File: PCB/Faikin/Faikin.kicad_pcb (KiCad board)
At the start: 2 copper layers, 70 x 70 mm, 47 parts, among them J1 1x5, J2 TC2030-USB-NL, J3 Reset, Q1 BSS138PS, U1 TPS562246, U4 ESP32-S3-MINI-1

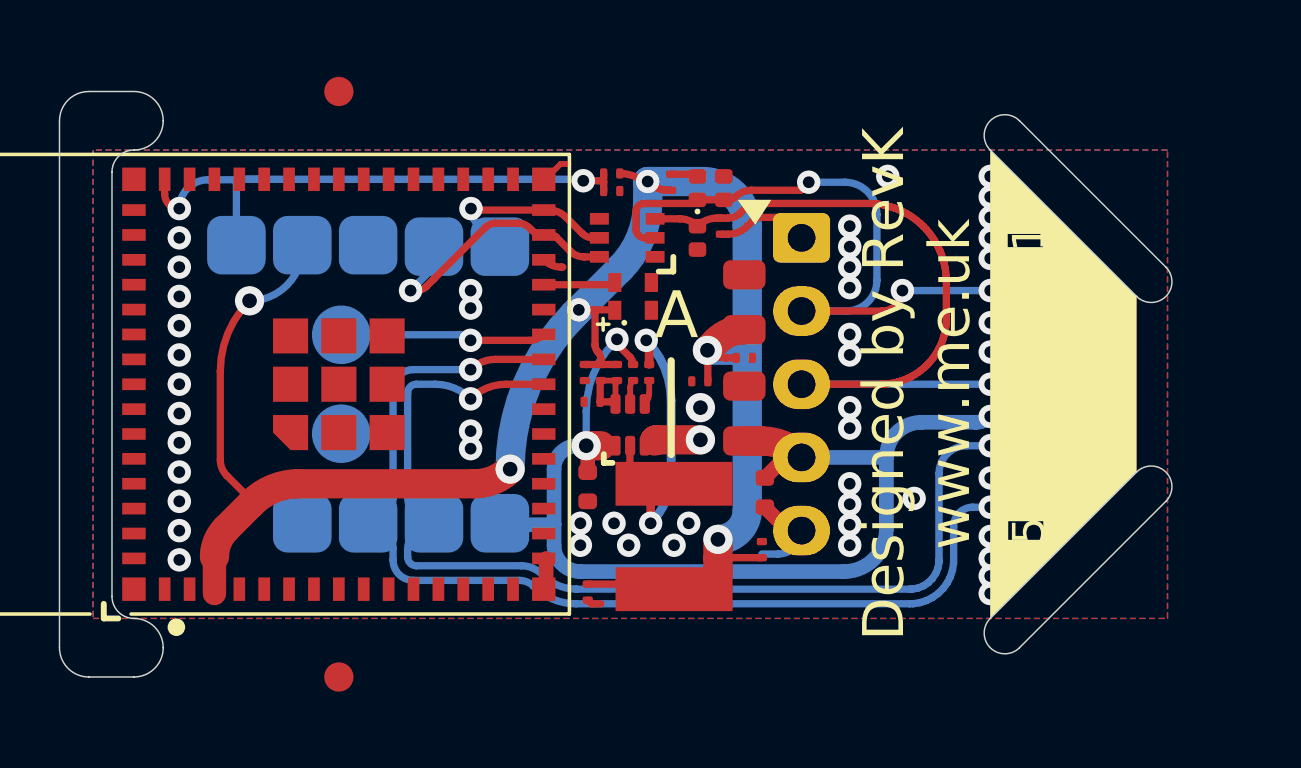
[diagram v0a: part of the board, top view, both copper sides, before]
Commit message: Minor tweaks
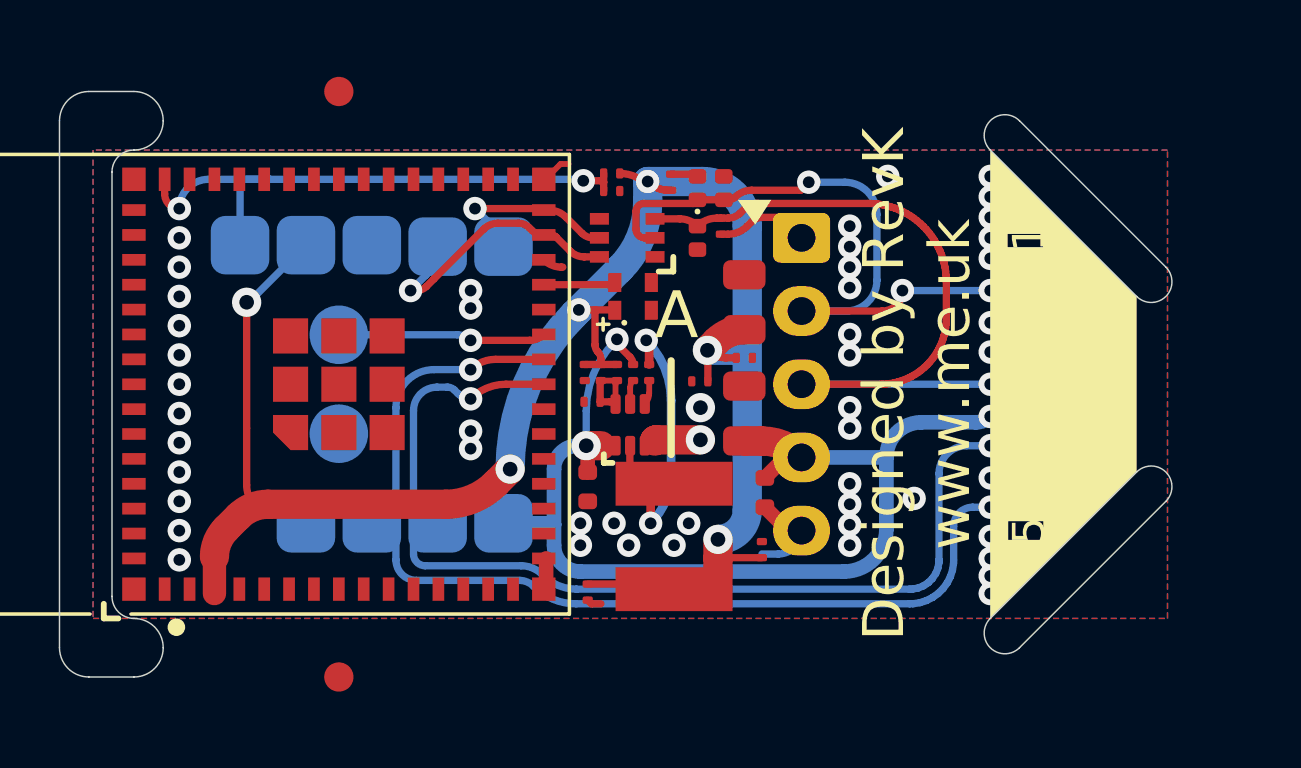
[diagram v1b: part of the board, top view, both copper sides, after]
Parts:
- D1: footprint RevK:SMD1615 -> RevK:SMD1615-Blind
- moved TP10 0.12 mm to (135.4, 60.3)
- moved TP2 0.12 mm to (133.1, 69.8)
- moved TP3 0.12 mm to (130.9, 69.8)
- moved TP4 0.12 mm to (128.6, 69.8)
- moved TP5 0.12 mm to (128.6, 60.2)
- moved TP6 0.12 mm to (126.4, 60.2)
- moved TP7 0.12 mm to (135.4, 69.8)
- moved TP8 0.12 mm to (130.9, 60.2)
- moved TP9 0.12 mm to (133.1, 60.3)
- moved J3 0.08 mm to (129.8, 65.0)
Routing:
- net D-: track 38.9 -> 37.2 mm
- net D+: track 43.7 -> 42.3 mm
- net TX: track 6.23 -> 5.34 mm
- net RX: track 8.62 -> 9.29 mm
- net +3.3V: track 65.8 -> 65.2 mm

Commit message: Library update
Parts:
- C15: value 47uF 6V -> 47uF 6V3
- D1: value XL-1516RGBC-WS2812B -> XL-1615RGBC-2812B
